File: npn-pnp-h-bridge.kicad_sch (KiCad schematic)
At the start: 90 parts, among them J1 S4B-PH-K-S_LF__SN_, J2 S2B-PH-K-S_LF__SN_, Q1 AO3400A, Q2 MMBT3904, Q3 AO3400A, Q4 MMBT3904

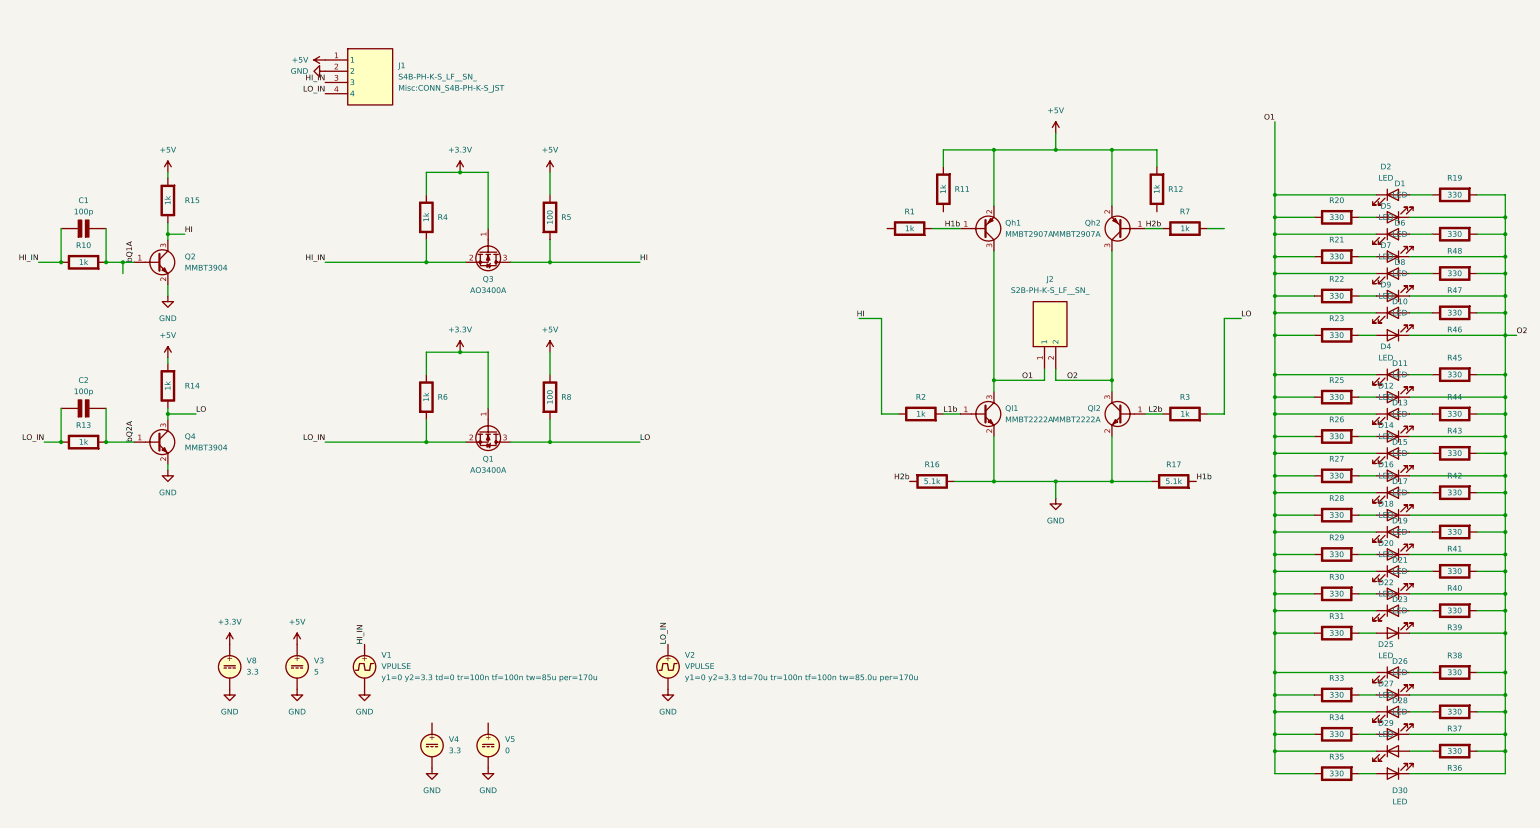
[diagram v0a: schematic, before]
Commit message: first appearently working prototype
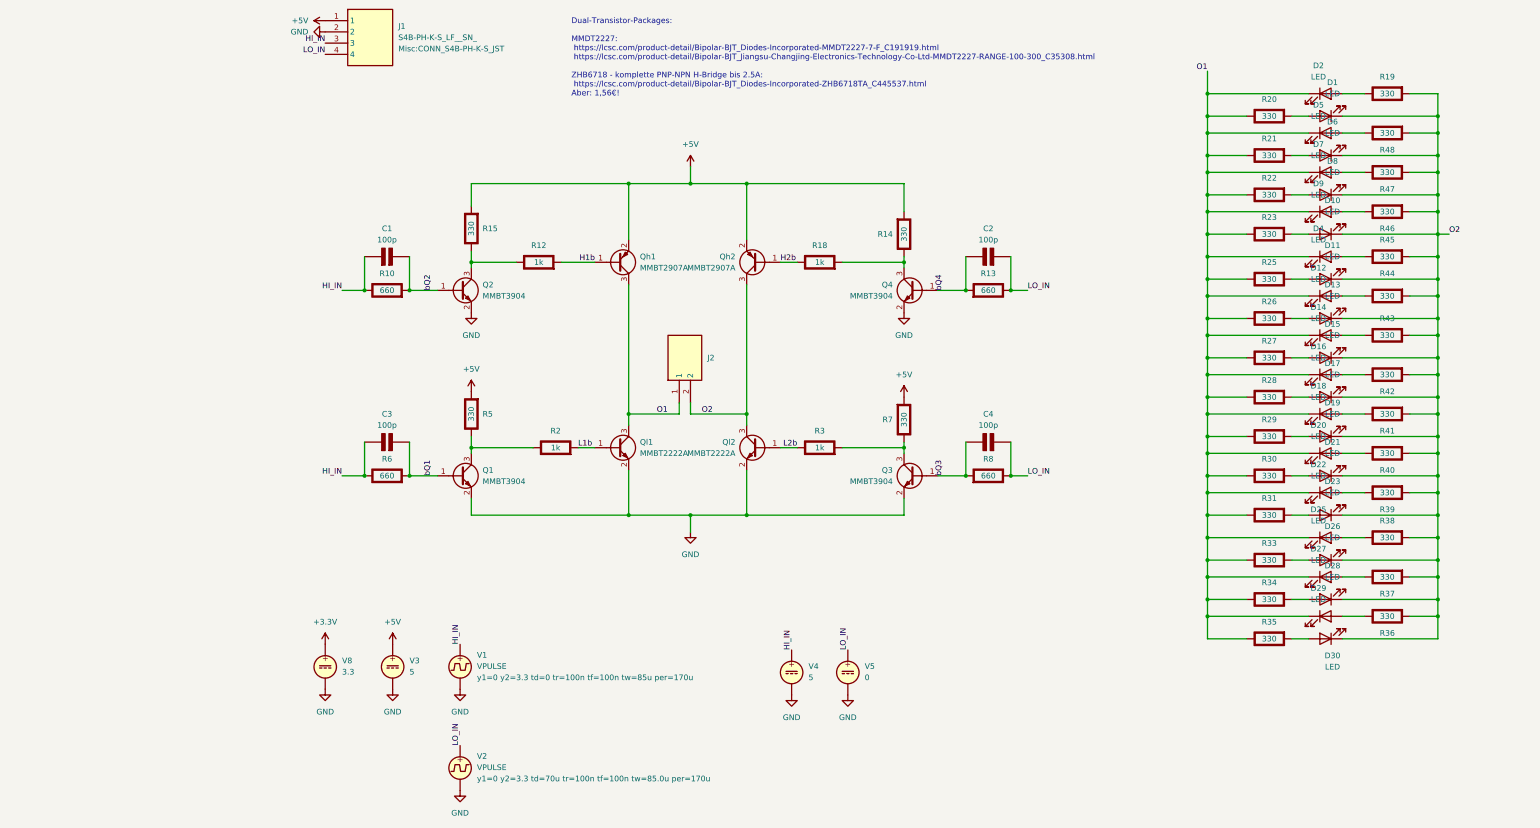
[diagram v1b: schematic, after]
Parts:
- removed Q1, Q3: AO3400A, Package_TO_SOT_SMD:SOT-23, symbol Transistor_FET:AO3400A
- removed R1, R11, R4: 1k, Resistor_SMD:R_0805_2012Metric_Pad1.20x1.40mm_HandSolder, symbol PCM_Elektuur:R
- removed R16, R17: 5.1k, Resistor_SMD:R_0805_2012Metric_Pad1.20x1.40mm_HandSolder, symbol PCM_Elektuur:R
- added C3, C4: 100p, Capacitor_SMD:C_0805_2012Metric_Pad1.18x1.45mm_HandSolder, symbol PCM_Elektuur:C
- added Q1, Q3: MMBT3904, Package_TO_SOT_SMD:SOT-23, symbol Transistor_BJT:MMBT3904
- added R18: 1k, Resistor_SMD:R_0805_2012Metric_Pad1.20x1.40mm_HandSolder, symbol PCM_Elektuur:R
- R10, R13, R6: value 1k -> 660
- R14, R15, R7: value 1k -> 330
- R5: value 100 -> 330
- R8: value 100 -> 660
- V4: value 3.3 -> 5
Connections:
- net +3.3V: no longer R6.1 (+)
- net +5V: now also R5.2 (-), R7.2 (-); no longer R12.2 (-), R5.1 (+), R8.1 (+)
- net GND: now also Q1.2 (E), Q3.2 (E)
- net H1b: now also R12.2 (-)
- net H2b: now also R18.1 (+); no longer R7.2 (-)
- net HI_IN: now also R6.1 (+), V4.1, C3.1 (+)
- net LO_IN: now also R8.1 (+), V5.1, C4.1 (+); no longer R6.2 (-)
- net at R12.1 (+): now also Q2.3 (C), R15.1 (+)
- net at R7.1 (+): now also R3.2 (-), Q3.3 (C)
- removed net HI : Q2.3 (C), R15.1 (+), R2.1 (+), R5.2 (-)
- net LO: no longer names the net of Q4.3 (C), R14.1 (+)
- net LO: now also R18.2 (-); no longer R3.2 (-), R8.2 (-)
- net bQ1A renamed bQ2
- net bQ2A renamed bQ4
- new net: Q1.3 (C), R2.1 (+), R5.1 (+)
- new net bQ1: C3.2 (-), Q1.1 (B), R6.2 (-)
- new net bQ3: C4.2 (-), Q3.1 (B), R8.2 (-)
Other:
- note added: "Dual-Transistor-Packages: MMDT2227: https://lcsc.com/product-detail/Bipolar-BJT_Diodes-Incorporated-MMDT2227-7-F_C191919.html https://lcsc.com/product-detail/Bipolar-BJT_Jiangsu-Changjing-Electronics-Technology-Co-Ltd-MMDT2227-RANGE-100-300_C35308.html ZHB6718 - komplette PNP-NPN H-Bridge bis 2.5A: https://lcsc.com/product-detail/Bipolar-BJT_Diodes-Incorporated-ZHB6718TA_C445537.html Aber: 1,56€!"
- moved on the sheet: C1, C2, D1, D10, D11, D12, D13, D14, D15, D16, D17, D18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
